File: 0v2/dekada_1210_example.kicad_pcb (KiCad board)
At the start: 2 copper layers, 49.8 x 33 mm, 43 parts, among them P1 CONN_02X10, P2 CONN_02X10, P3 CONN_02X10, P4 CONN_02X10, P5 CONN_01X02, P6 CONN_01X02, P7 CONN_01X02

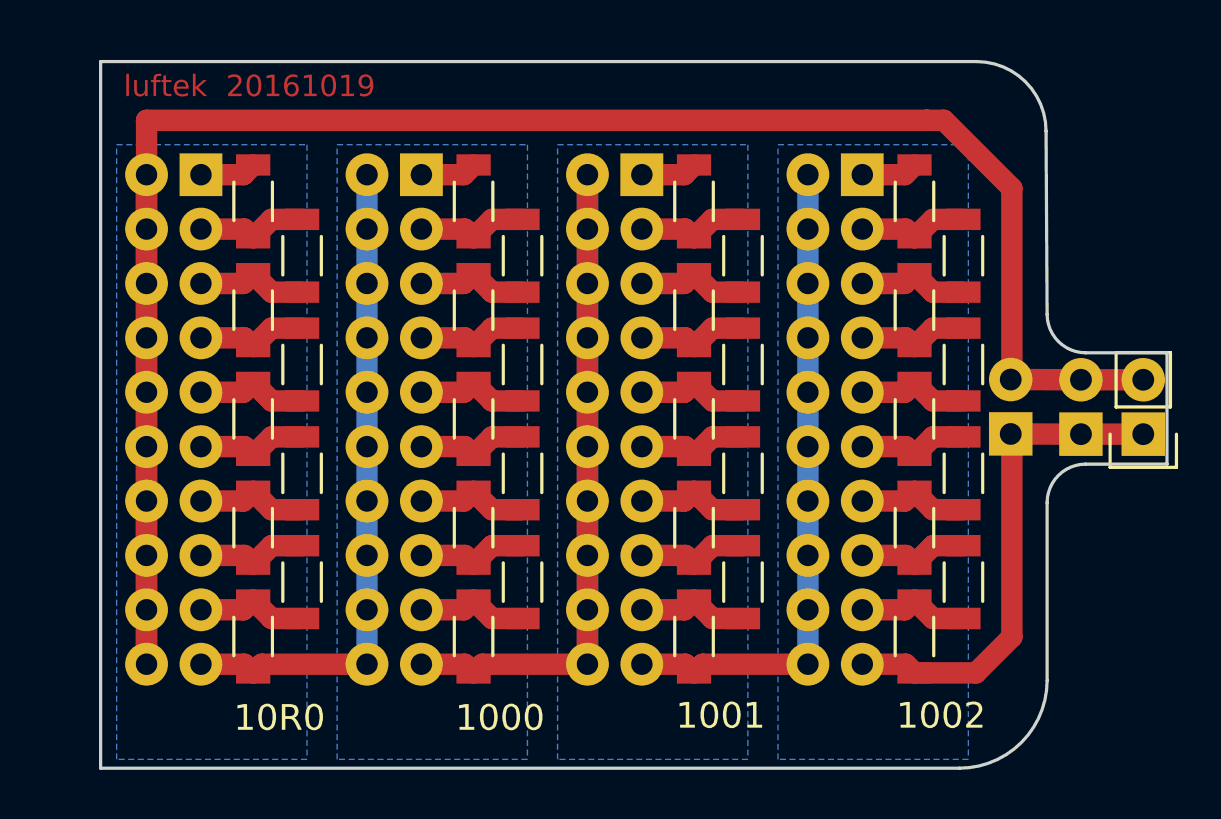
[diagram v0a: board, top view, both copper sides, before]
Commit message: Version 0v3
assembled, tested, working
no downsides or need for improvement found for now
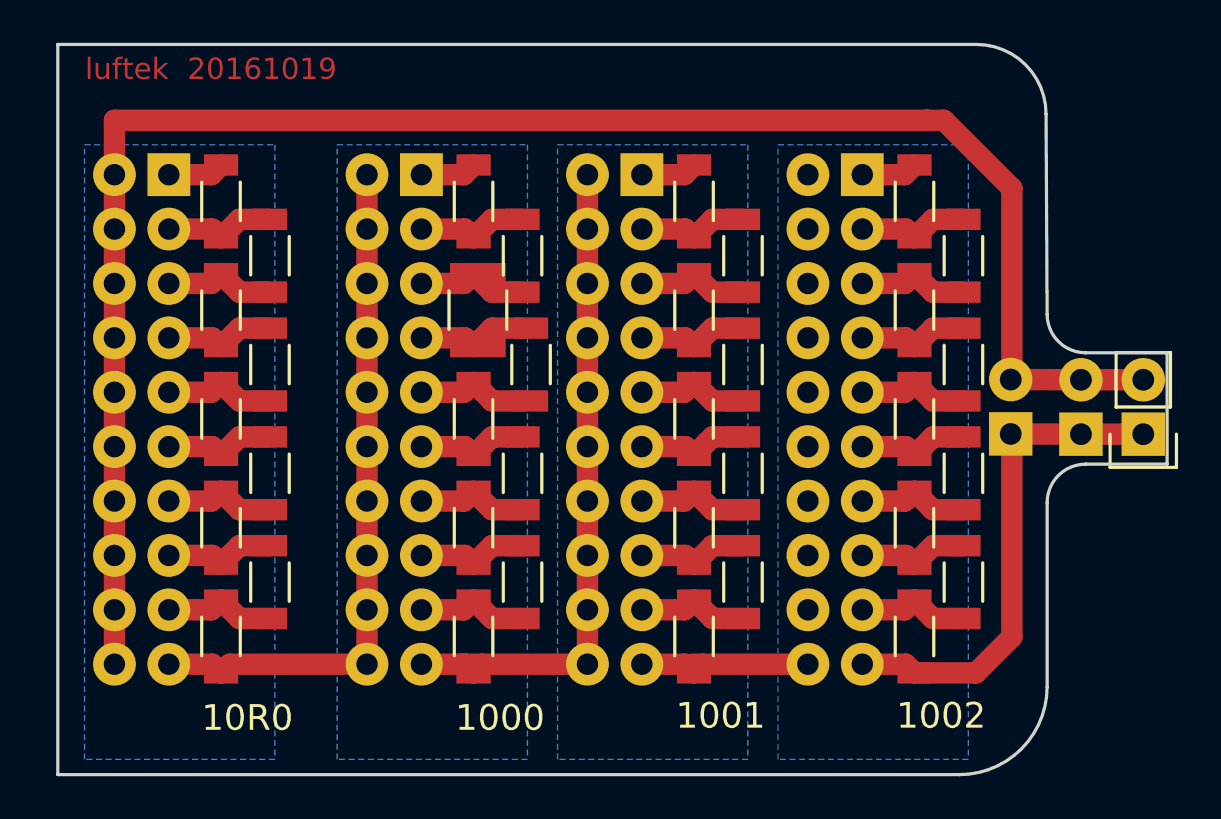
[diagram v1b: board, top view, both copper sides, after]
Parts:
- R13: footprint R_1206_Custom -> R_1210_Custom
- moved P1 1.50 mm to (86.9, 33.6)
- moved R1 1.50 mm to (89.3, 34.8)
- moved R2 1.50 mm to (91.6, 37.4)
- moved R3 1.50 mm to (89.3, 39.9)
- moved R4 1.50 mm to (91.6, 42.5)
- moved R5 1.50 mm to (89.3, 45.0)
- moved R6 1.50 mm to (91.6, 47.5)
- moved R7 1.50 mm to (89.3, 50.1)
- moved R8 1.50 mm to (91.6, 52.6)
- moved R9 1.50 mm to (89.3, 55.2)
- moved R14 0.40 mm to (103.8, 42.5)
- moved R13 0.20 mm to (101.3, 39.9)
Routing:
- net Net-(P3-Pad19): track 31.0 -> 8.59 mm
- net Net-(P2-Pad19): track 53.8 -> 31.5 mm
- net Net-(P1-Pad10): track 105.4 -> 84.0 mm
- net Net-(P1-Pad19): track 31.0 -> 31.5 mm
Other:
- board size 49.8 x 33 mm -> 51.8 x 34.1 mm
